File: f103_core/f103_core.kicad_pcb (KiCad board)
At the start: 2 copper layers, 53.3 x 30.5 mm, 29 parts, among them J1 Conn_02x20_Odd_Even, J4 Conn_01x04, J5 Conn_02x03_Odd_Even, SW1 SW_Push, U1 STM32F103C6Tx, U2 AMS1117-3.3, Y1 8M, Y2 32.768

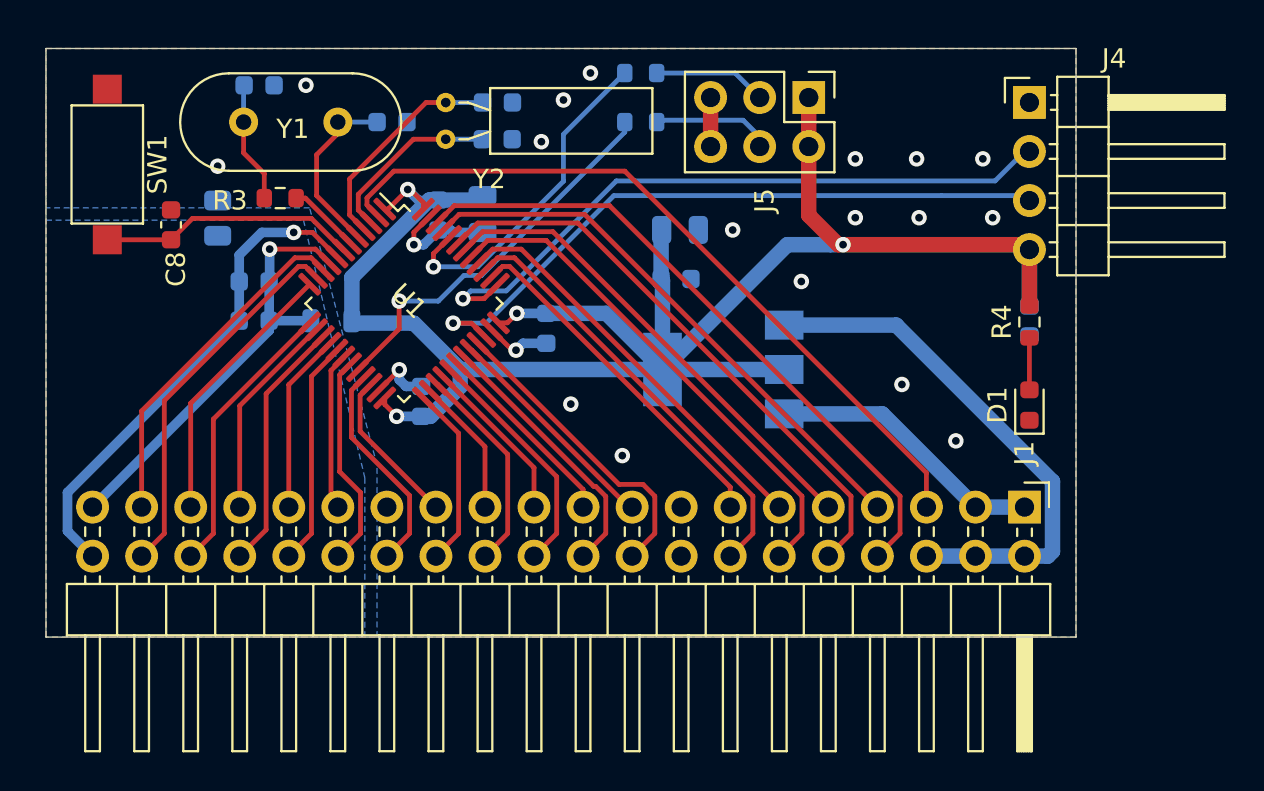
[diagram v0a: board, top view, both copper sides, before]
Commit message: Update pcb for f103_core.
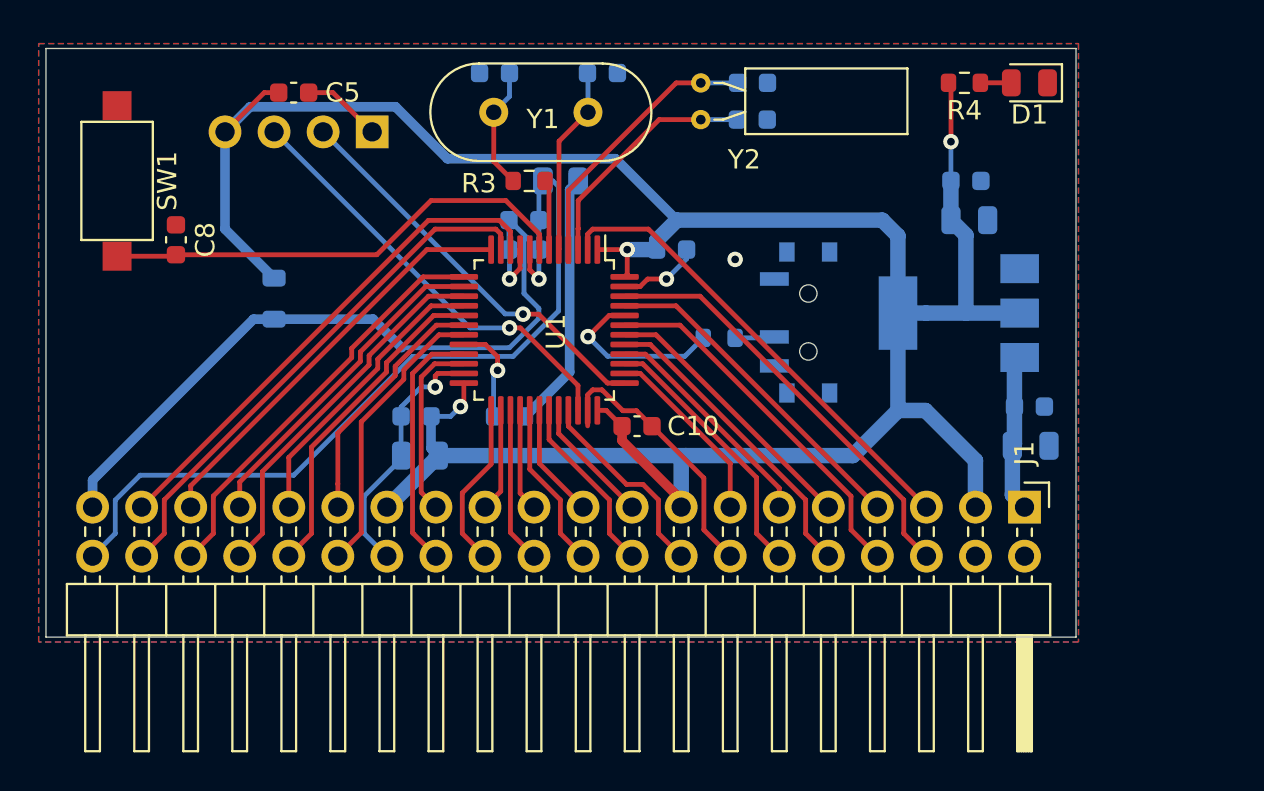
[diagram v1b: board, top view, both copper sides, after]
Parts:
- removed J5: Conn_02x03_Odd_Even, Connector_PinHeader_2.54mm:PinHeader_2x03_P2.54mm_Vertical
- added C15: 10uF, Capacitor_SMD:C_0805_2012Metric, B.Cu at (154.5, 126.0)
- added C16: 100nF, Capacitor_SMD:C_0603_1608Metric, B.Cu at (154.4, 124.0)
- added SW2: SW_DPDT_x2, Button_Switch_SMD:SW_SPDT_PCM12, B.Cu at (142.7, 119.6)
- C10, C5: moved to F.Cu
- D1: footprint LED_SMD:LED_0603_1608Metric -> LED_SMD:LED_0805_2012Metric
- J4: moved to B.Cu
- moved C5 39.9 mm to (116.3, 107.7), turned to 0 degrees
- moved J4 34.1 mm to (120.4, 109.7), turned to 90 degrees
- moved R5 17.9 mm to (130.2, 112.3), turned to 180 degrees
- moved R2 16.7 mm to (127.5, 124.5)
- moved D1 16.7 mm to (154.4, 107.2), turned to 180 degrees
- moved C7 15.8 mm to (151.1, 112.3)
- moved C9 15.2 mm to (135.9, 115.8), turned to 0 degrees
- moved C6 15.0 mm to (151.3, 114.3)
- moved C14 14.4 mm to (128.3, 115.8), turned to 0 degrees
- moved C13 14.3 mm to (128.3, 114.3), turned to 0 degrees
- moved R1 14.3 mm to (138.4, 120.4)
- moved C4 13.2 mm to (140.1, 107.2)
- moved C3 13.2 mm to (140.1, 109.1)
- moved Y2 13.2 mm to (137.4, 109.1)
- moved Y1 13.0 mm to (131.6, 108.7)
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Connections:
- J1 pad 10: /PB7 -> /PB5
- J1 pad 12: /PB5 -> /PB3
- J1 pad 14: /PB3 -> GND
- J1 pad 15: /PF6 -> +3V3
- J1 pad 16: /PF7 -> /PA12
- J1 pad 18: /PA12 -> /PA10
- J1 pad 20: /PA10 -> /PA8
- J1 pad 22: /PA8 -> /PB14
- J1 pad 24: /PB14 -> /PB12
- J1 pad 26: /PB12 -> /PB10
- J1 pad 27: /PB2 -> +3V3
- J1 pad 28: /PB10 -> GND
- J1 pad 3: VCC -> +3V3
- J1 pad 6: GND -> /PB9
- J1 pad 8: /PB9 -> /PB7
- R2 pad 2: Net-(J5-Pad4) -> GND
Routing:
- net +3V3: track 108.6 -> 135.9 mm, vias 4 -> 3
- net GNDA: track 25.9 -> 44.7 mm
- net +3.3VA: track 22.8 -> 39.9 mm
- net /BOOT1: track 20.3 -> 5.19 mm
- net /PC13: track 39.0 -> 24.4 mm
- net /SYS_JTCK-SWCL: track 34.7 -> 21.2 mm
- net /SYS_JTMS-SWDIO: track 34.5 -> 22.5 mm
- net /PB9: track 34.2 -> 22.2 mm
- net /PB8: track 29.1 -> 17.4 mm
- net /PB7: track 30.3 -> 19.1 mm
- net RESET: track 13.4 -> 24.6 mm
- net /PB6: track 25.2 -> 14.2 mm
- net /PB5: track 26.6 -> 16.1 mm
- net /PB4: track 21.5 -> 11.9 mm
- net /PB3: track 22.9 -> 13.8 mm
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- removed copper zone on B.Cu, net GNDA
